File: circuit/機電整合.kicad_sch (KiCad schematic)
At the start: 7 parts, among them U1 L293D, U2 74HC595, U3 74HC595, U4 L293D, U5 L293D, U6 ESP32-CAM

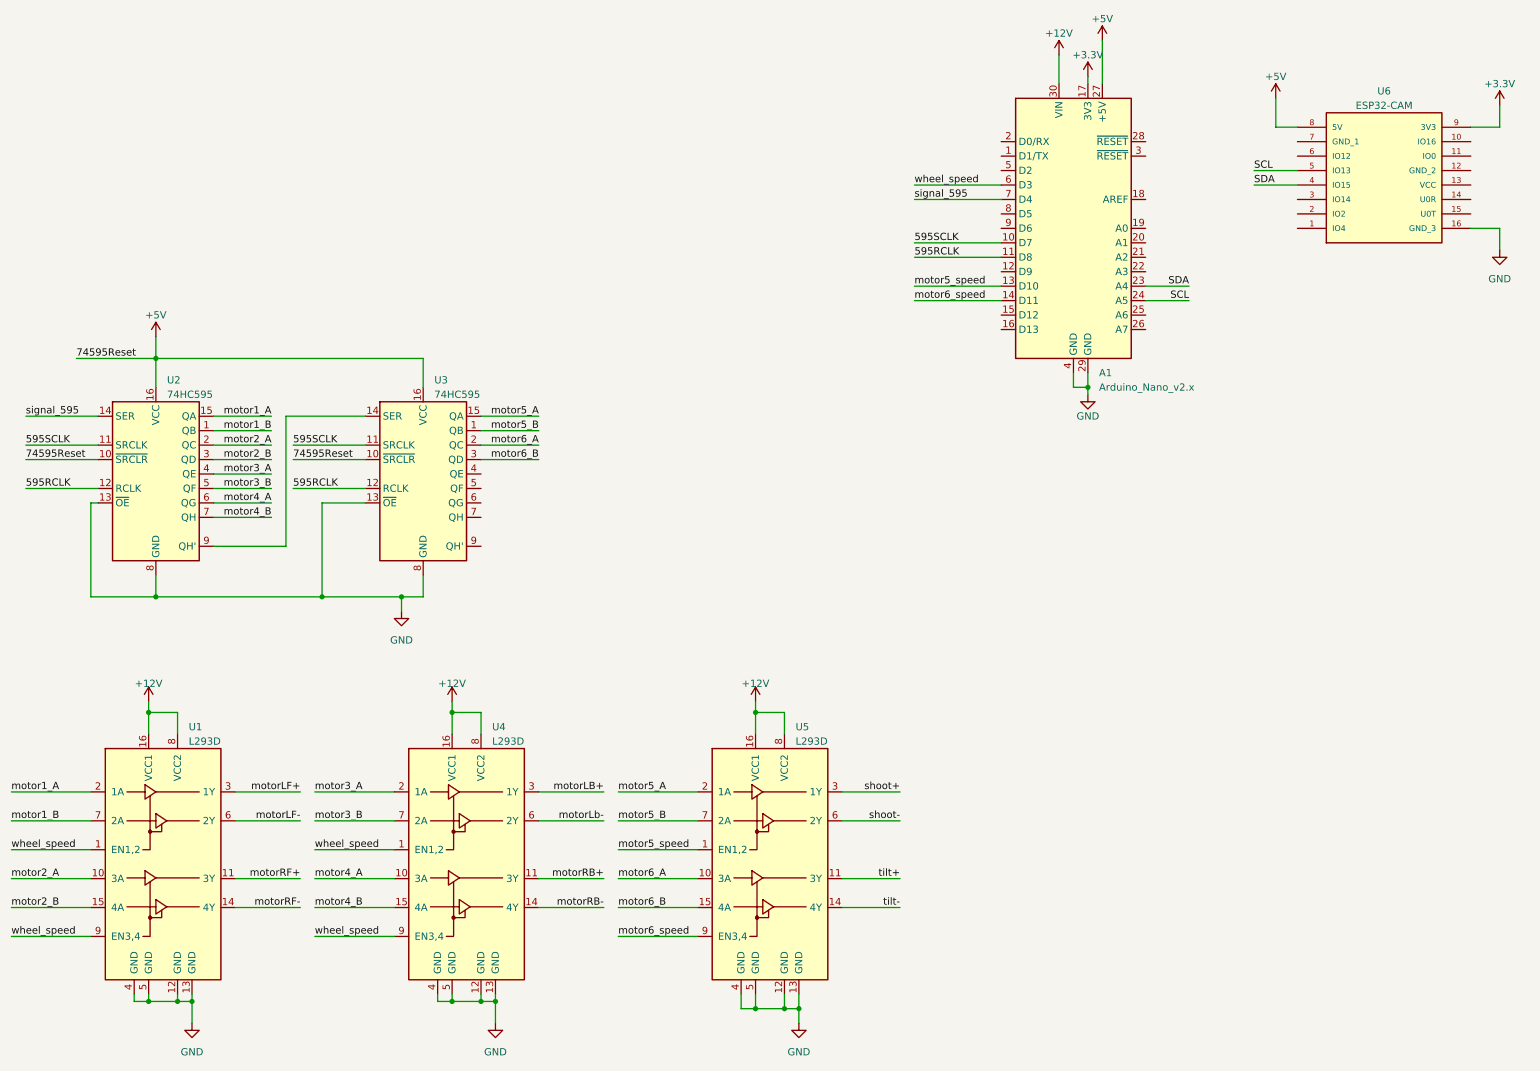
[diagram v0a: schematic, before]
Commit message: update circuit diagram
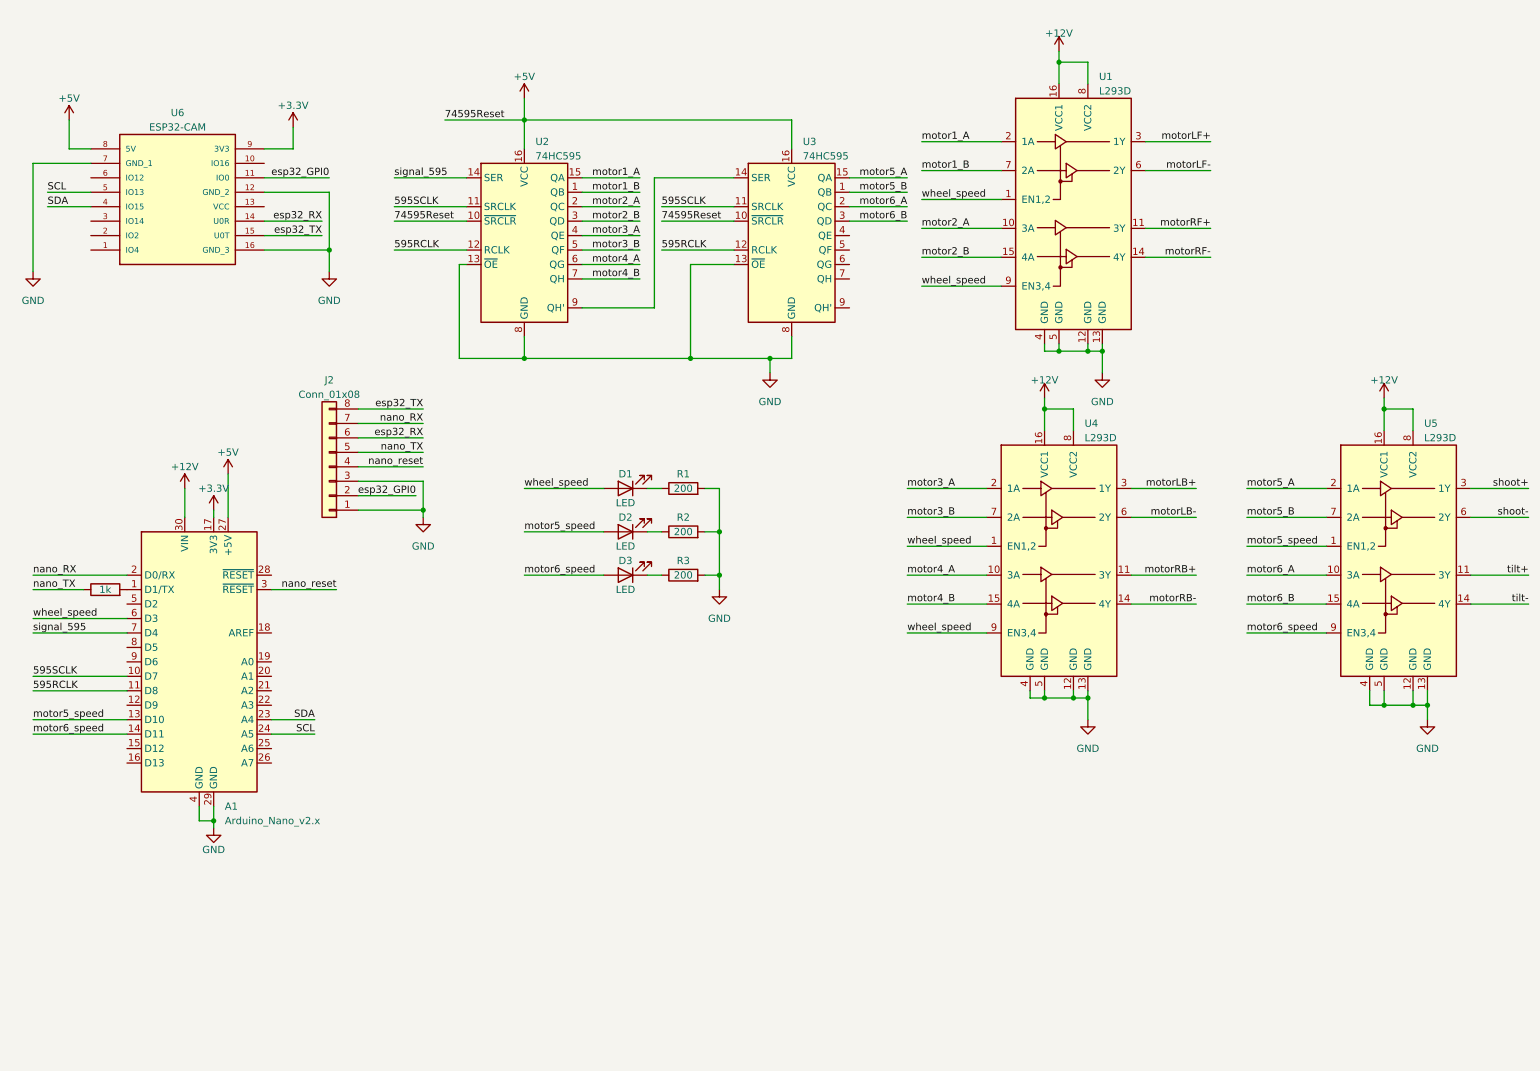
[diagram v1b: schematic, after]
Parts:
- added D1, D2, D3: LED, LED_THT:LED_D3.0mm_FlatTop, symbol Device:LED
- added J2: Conn_01x08, Connector_PinHeader_2.54mm:PinHeader_1x08_P2.54mm_Vertical, symbol Connector_Generic:Conn_01x08
- added R1, R2, R3: 200, LED_THT:LED_D3.0mm_FlatTop, symbol Device:R
- added R4: 1k, symbol Device:R
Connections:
- net GND: now also U6.12 (GND_2), U6.7 (GND_1), J2.1 (Pin_1), J2.3 (Pin_3), R1.2, R2.2, R3.2
- net motor5_speed: now also D2.2 (A)
- net motor6_speed: now also D3.2 (A)
- net wheel_speed: now also D1.2 (A)
- net at A1.1 (D1/TX): now also R4.2
- net nano_RX: now reaches A1.2 (D0/RX)
- net nano_RX: now also J2.7 (Pin_7)
- net nano_reset: now reaches A1.3 (~{RESET})
- net nano_reset: now also J2.4 (Pin_4)
- net esp32_GPI0: now reaches U6.11 (IO0)
- net esp32_GPI0: now also J2.2 (Pin_2)
- net esp32_RX: now reaches U6.14 (U0R)
- net esp32_RX: now also J2.6 (Pin_6)
- net esp32_TX: now reaches U6.15 (U0T)
- net esp32_TX: now also J2.8 (Pin_8)
- net motorLb- renamed motorLB-
- new net: D3.1 (K), R3.1
- new net: D2.1 (K), R2.1
- new net: D1.1 (K), R1.1
- new net nano_TX: J2.5 (Pin_5), R4.1
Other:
- moved on the sheet: A1, U1, U2, U3, U4, U5, U6
